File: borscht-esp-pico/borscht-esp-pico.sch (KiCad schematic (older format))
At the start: 25 parts, among them J1 USB, J2 GPIO, J3 GPIO, Q1 S8050, Q2 S8050, U1 ESP32-PICO-D4, U2 ESP-PSRAM32, U3 CH340C, U4 AZ1117-3.3

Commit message: Add reset/reboot buttons
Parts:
- removed AE1: Antenna, AN9520:SMD_ANT9520, symbol Device:Antenna
- added ANT1: AN9520, AN9520:SMD_ANT9520, symbol AN9520:AN9520
- added C9: 0.1uF, symbol Device:C
- added SW1: BOOT, symbol Switch:SW_Push
- added SW2: RESET, symbol Switch:SW_Push
- U4: value AZ1117-3.3 -> AMS1117; footprint Package_TO_SOT_SMD:SOT-223 -> Package_TO_SOT_SMD:SOT-223-3_TabPin2; symbol Regulator_Linear:AZ1117-3.3 -> Regulator_Linear:AMS1117-3.3
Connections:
- net EN: now also C9.2, SW2.1
- net GND: now also C9.1, SW1.2, SW2.2
- net IO0: now also SW1.1
- net at U1.2 (LNA_IN): now also ANT1.P$FEED
- no-connect marks 11 -> 12
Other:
- moved on the sheet: C1, C2, C3, C4, C7, C8, D1, J2, J3, Q1, R1, R2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

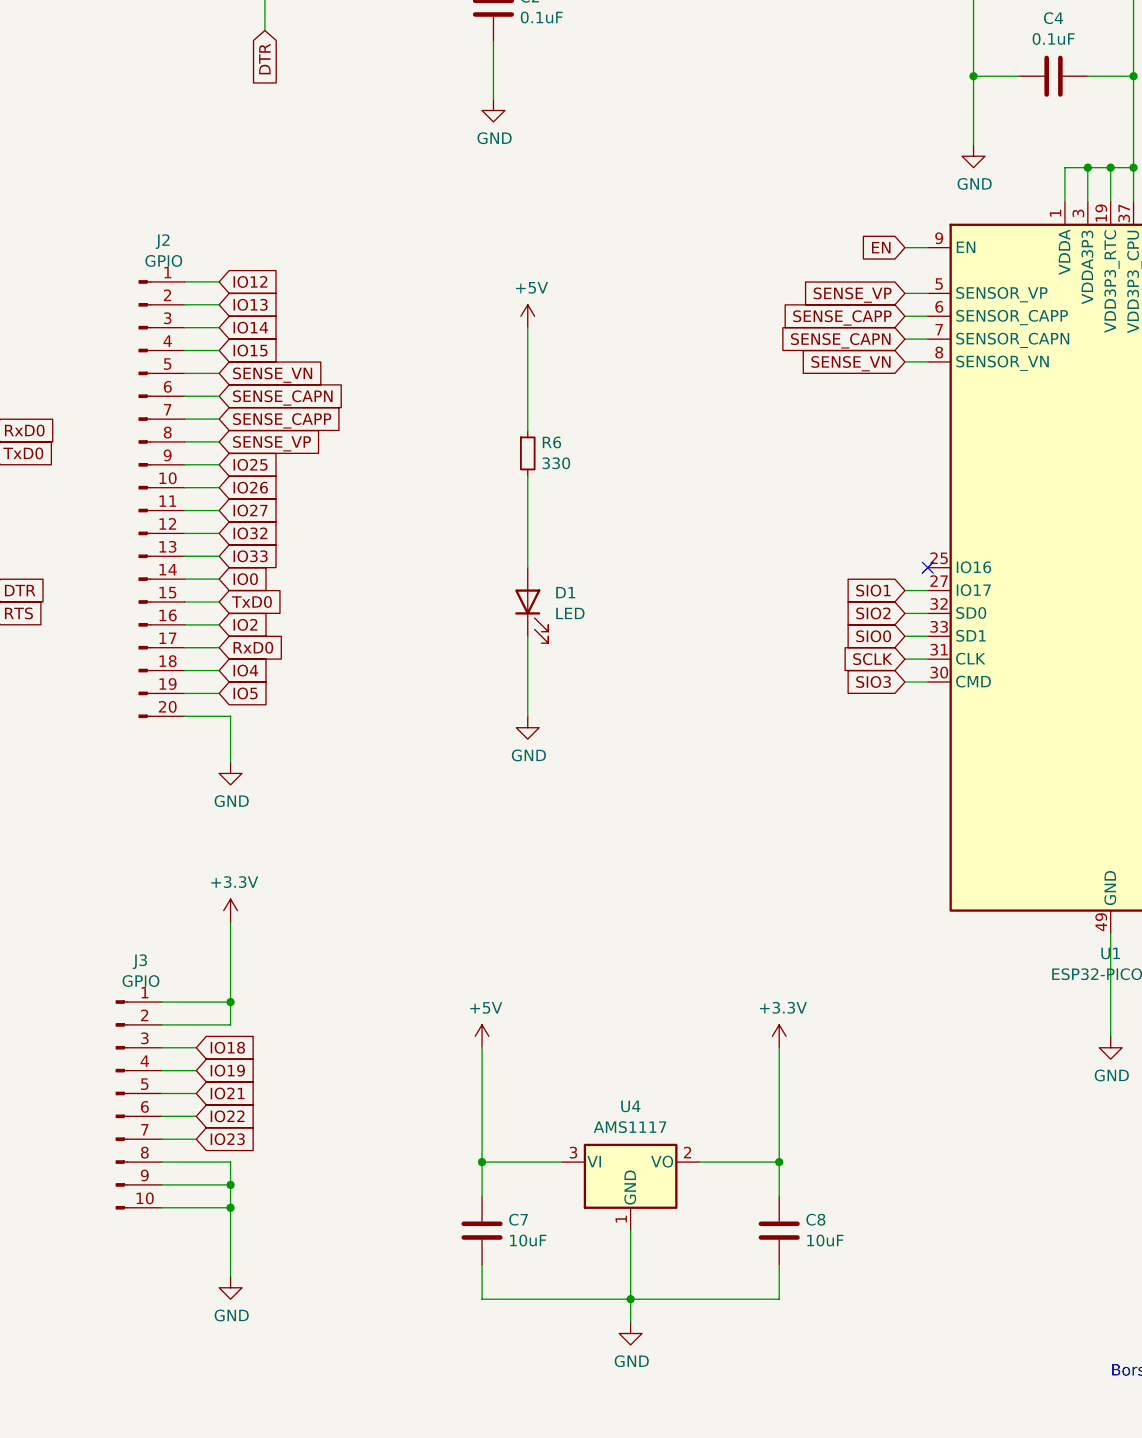
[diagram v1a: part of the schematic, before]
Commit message: Add PCB Rev 1
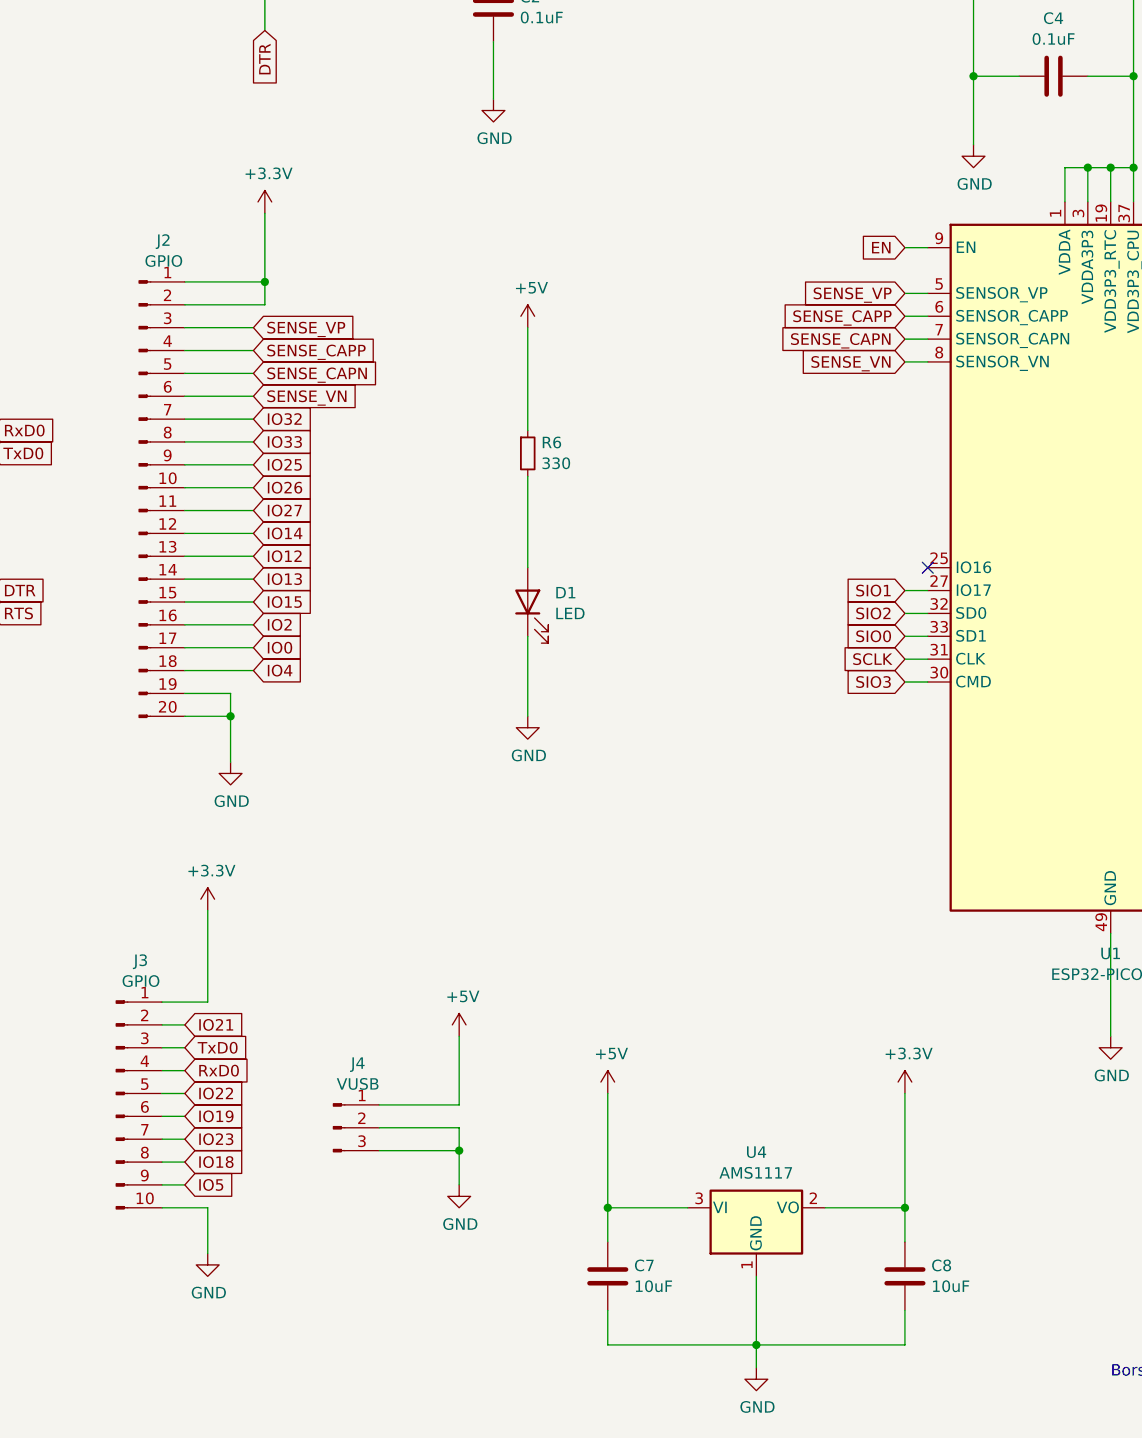
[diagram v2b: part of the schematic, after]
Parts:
- added J4: VUSB, Connector_PinSocket_2.54mm:PinSocket_1x03_P2.54mm_Vertical, symbol Connector:Conn_01x03_Male
- C9: footprint (none) -> Capacitor_SMD:C_0603_1608Metric_Pad1.05x0.95mm_HandSolder
- Q1, Q2: footprint Package_TO_SOT_THT:TO-92_Inline -> Package_TO_SOT_SMD:SOT-23
- SW1, SW2: footprint (none) -> Button_Switch_SMD:SW_SPST_REED_CT05-XXXX-J1
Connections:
- net +3V3: now also J2.1 (Pin_1), J2.2 (Pin_2); no longer J3.2 (Pin_2)
- net +5V: now also J4.1 (Pin_1)
- net GND: now also J2.19 (Pin_19), J4.2 (Pin_2), J4.3 (Pin_3); no longer J3.8 (Pin_8), J3.9 (Pin_9)
- net IO0: now also J2.17 (Pin_17); no longer J2.14 (Pin_14)
- net IO12: now also J2.13 (Pin_13); no longer J2.1 (Pin_1)
- net IO13: now also J2.14 (Pin_14); no longer J2.2 (Pin_2)
- net IO14: now also J2.12 (Pin_12); no longer J2.3 (Pin_3)
- net IO15: now also J2.15 (Pin_15); no longer J2.4 (Pin_4)
- net IO18: now also J3.8 (Pin_8); no longer J3.3 (Pin_3)
- net IO19: now also J3.6 (Pin_6); no longer J3.4 (Pin_4)
- net IO21: now also J3.2 (Pin_2); no longer J3.5 (Pin_5)
- net IO22: now also J3.5 (Pin_5); no longer J3.6 (Pin_6)
- net IO32: now also J2.7 (Pin_7); no longer J2.12 (Pin_12)
- net IO33: now also J2.8 (Pin_8); no longer J2.13 (Pin_13)
- net IO5: now also J3.9 (Pin_9); no longer J2.19 (Pin_19)
- net RxD0: now also J3.4 (Pin_4); no longer J2.17 (Pin_17)
- net SENSE_CAPN: now also J2.5 (Pin_5); no longer J2.6 (Pin_6)
- net SENSE_CAPP: now also J2.4 (Pin_4); no longer J2.7 (Pin_7)
- net SENSE_VN: now also J2.6 (Pin_6); no longer J2.5 (Pin_5)
- net SENSE_VP: now also J2.3 (Pin_3); no longer J2.8 (Pin_8)
- net TxD0: now also J3.3 (Pin_3); no longer J2.15 (Pin_15)
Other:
- moved on the sheet: C7, C8, U4
